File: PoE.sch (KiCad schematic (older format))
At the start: 25 parts, among them IC1 TPS2378DDA

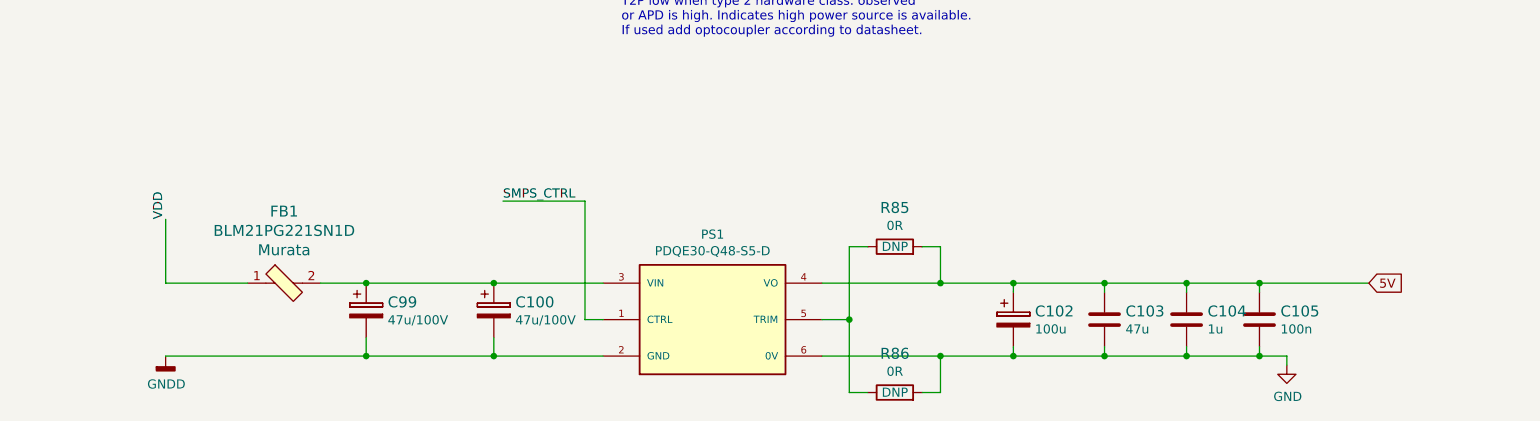
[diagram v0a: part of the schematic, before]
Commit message: annotations
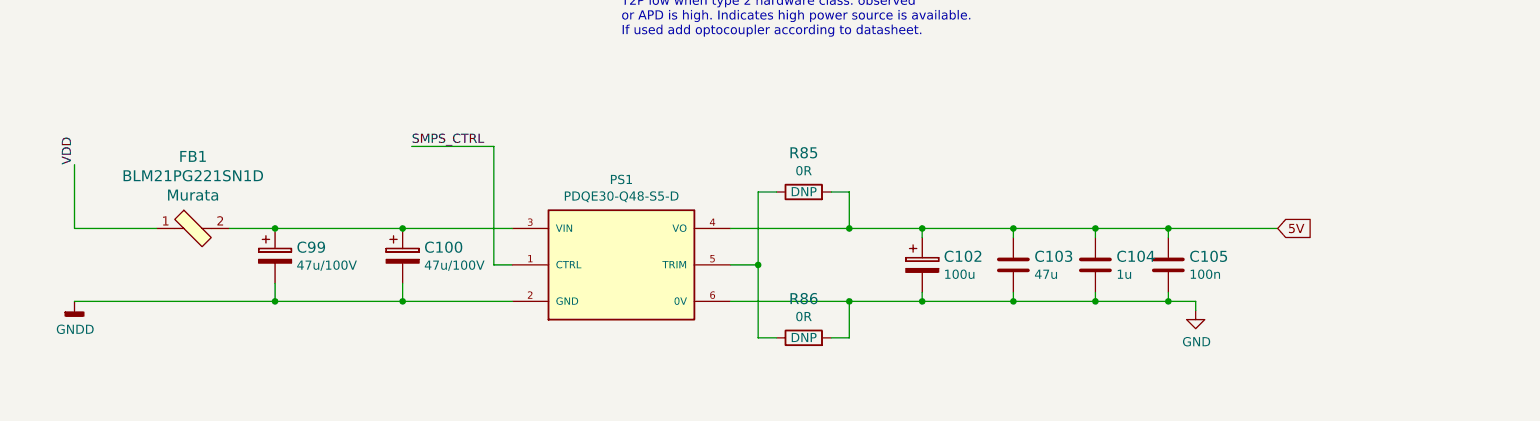
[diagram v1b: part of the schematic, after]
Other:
- moved on the sheet: C100, C102, C103, C104, C105, C99, FB1, PS1, R85, R86
